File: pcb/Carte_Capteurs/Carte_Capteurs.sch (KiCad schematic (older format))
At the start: 17 parts, among them J10 Conn_01x05, J11 Conn_01x04, J12 Conn_01x04, J5 Conn_02x07_Odd_Even, J6 Molex KK 254, J7 Samtec FTS-105-01-L-DV, J8 Samtec FTS-105-01-L-DV, J9 Conn_01x05, U1 FRDM-KL25Z, U2 XBee

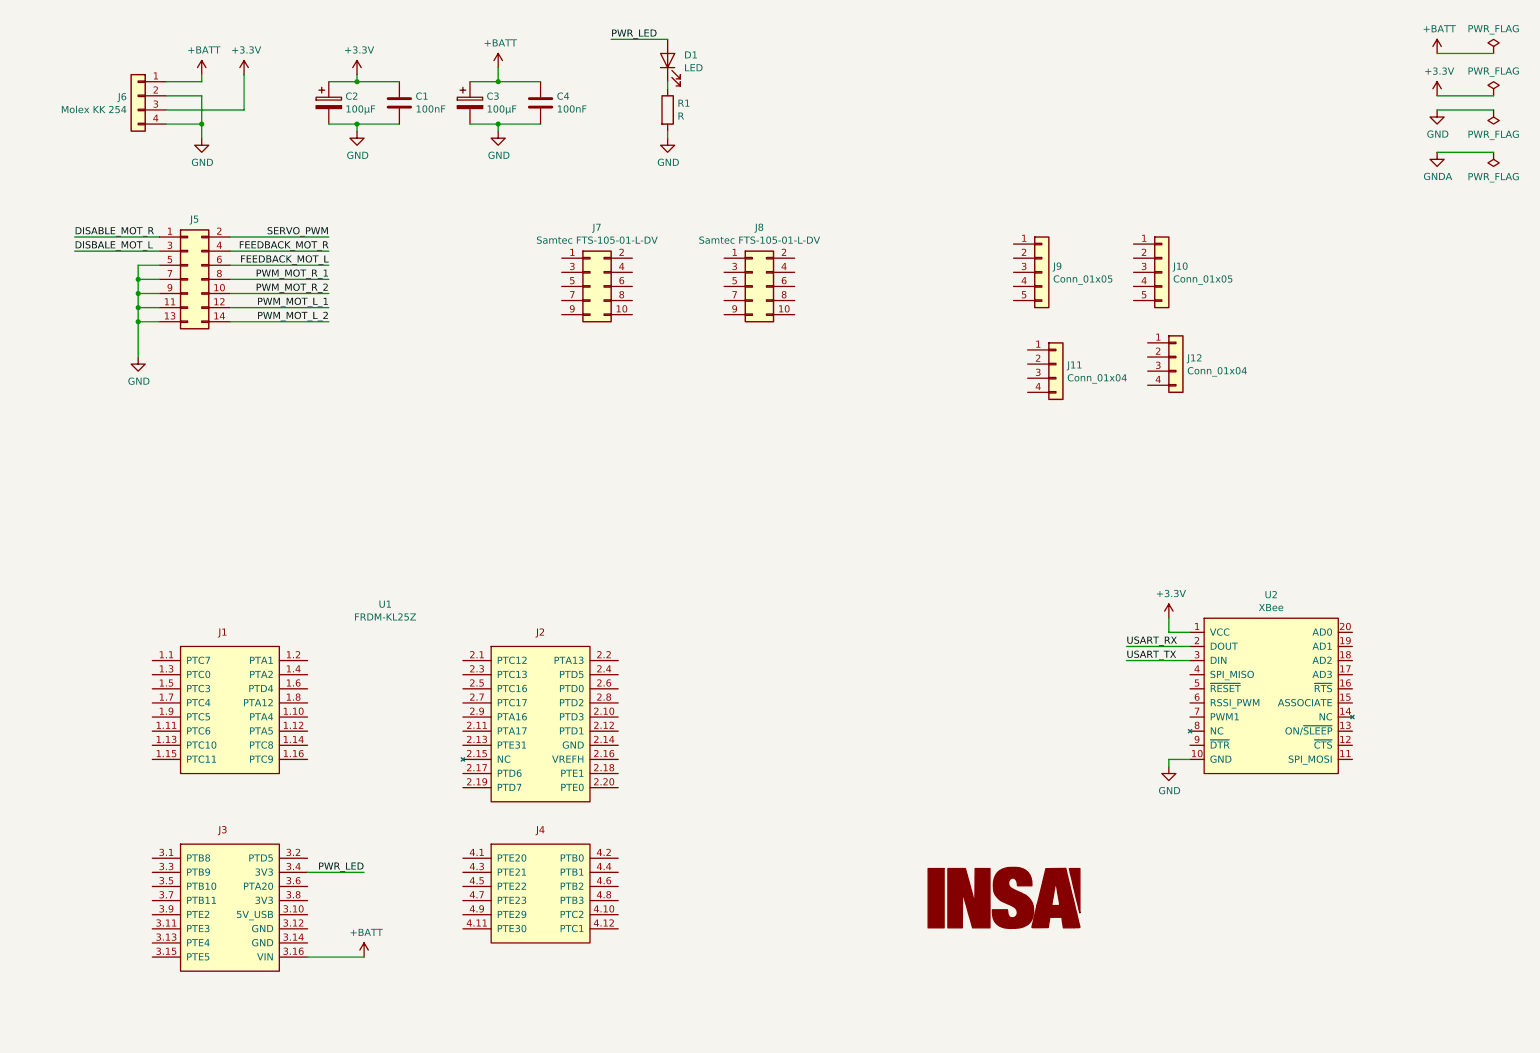
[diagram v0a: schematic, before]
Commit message: sauvegarde intermediaire
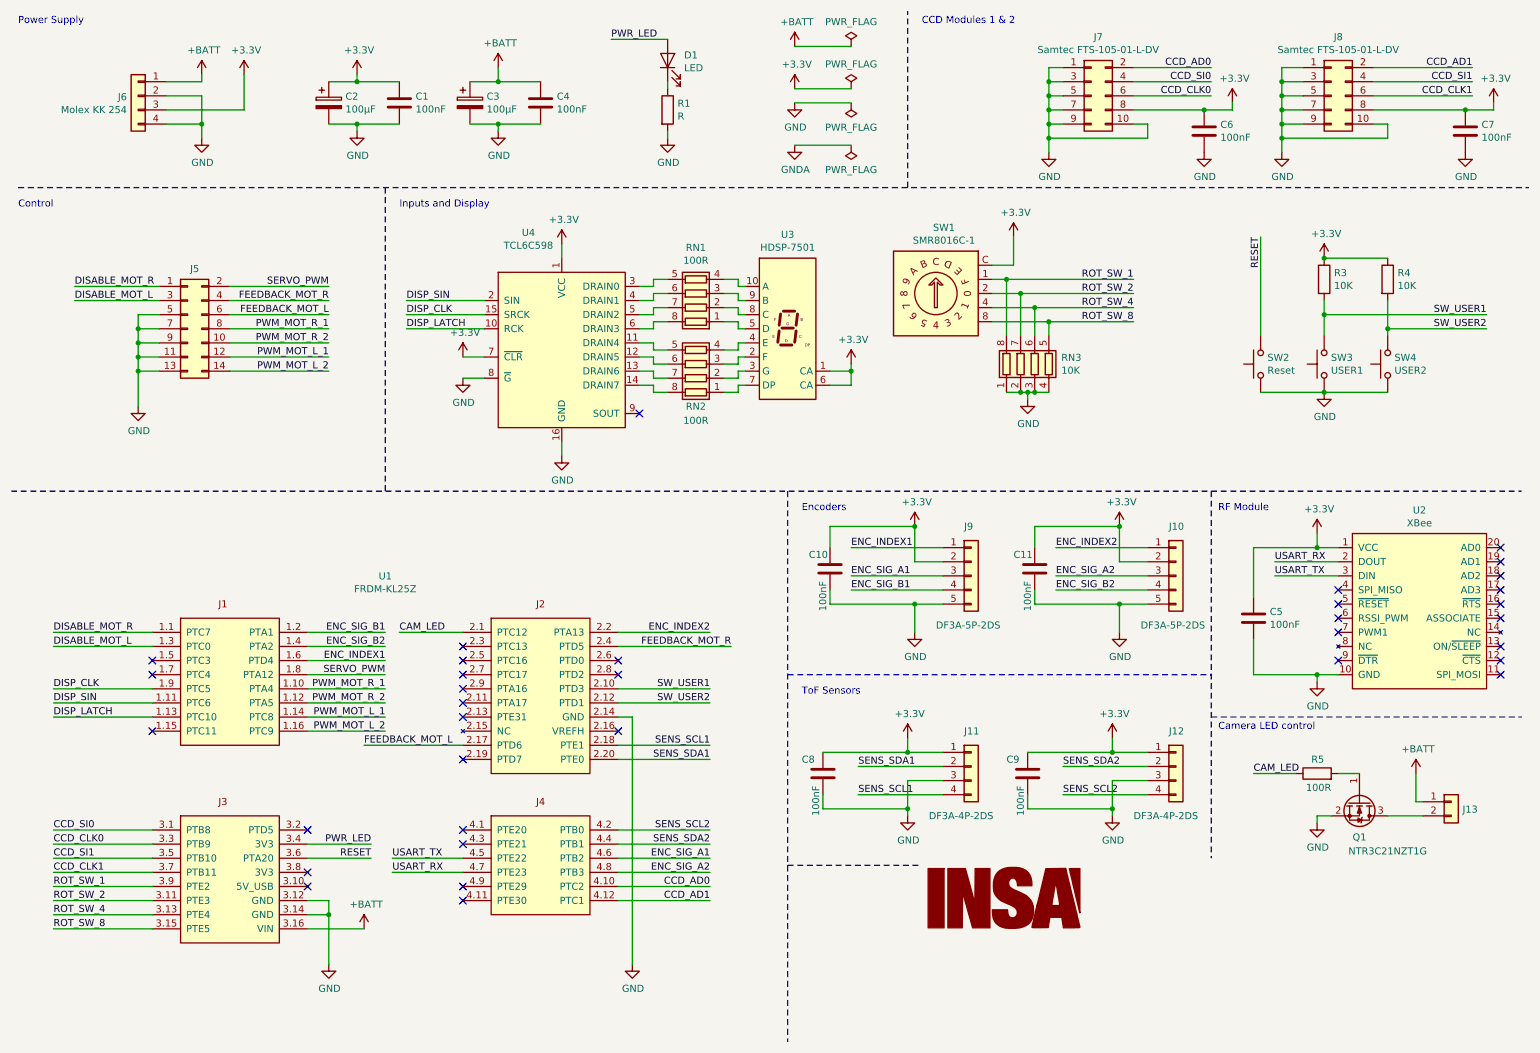
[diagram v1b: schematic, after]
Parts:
- added C10, C11, C5, C6, C7, C8, C9: 100nF, Capacitor_SMD:C_1206_3216Metric_Pad1.42x1.75mm_HandSolder, symbol Device:C
- added J13: Conn_01x02, Connector_PinHeader_2.54mm:PinHeader_1x02_P2.54mm_Vertical, symbol Connector_Generic:Conn_01x02
- added Q1: NTR3C21NZT1G, Package_TO_SOT_SMD:SOT-23, symbol Device:Q_NMOS_GSD
- added R3, R4: 10K, Resistor_SMD:R_1206_3216Metric_Pad1.42x1.75mm_HandSolder, symbol Device:R
- added R5: 100R, Resistor_SMD:R_1206_3216Metric_Pad1.42x1.75mm_HandSolder, symbol Device:R
- added RN1, RN2: 100R, Resistor_SMD:R_Array_Convex_4x1206, symbol Device:R_Pack04
- added RN3: 10K, Resistor_SMD:R_Array_Convex_4x1206, symbol Device:R_Pack04
- added SW1: SMR8016C-1, Insa:Nidec_Copal_SMR-8016C, symbol Switch:SW_Coded_SH-7050
- added SW2: Reset, Button_Switch_THT:SW_PUSH_6mm_H4.3mm, symbol Switch:SW_Push
- added SW3: USER1, Button_Switch_THT:SW_PUSH_6mm_H4.3mm, symbol Switch:SW_Push
- added SW4: USER2, Button_Switch_THT:SW_PUSH_6mm_H4.3mm, symbol Switch:SW_Push
- added U3: HDSP-7501, Display_7Segment:HDSP-A151, symbol Display_Character:HDSP-7501
- added U4: TCL6C598, Package_SO:TSSOP-16_4.4x5mm_P0.65mm, symbol Insa:TCL6C598
- J10, J9: value Conn_01x05 -> DF3A-5P-2DS; footprint Connector_PinHeader_2.54mm:PinHeader_1x05_P2.54mm_Horizontal -> Insa:DF3A-5P-2DS
- J11, J12: value Conn_01x04 -> DF3A-4P-2DS; footprint Connector_PinHeader_2.54mm:PinHeader_1x04_P2.54mm_Horizontal -> Insa:DF3A-4P-2DS
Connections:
- net DISBALE_MOT_L is gone; now on net DISABLE_MOT_L: J5.3 (Pin_3)
- net +3V3: now also J10.2 (Pin_2), J11.1 (Pin_1), J12.1 (Pin_1), J7.8 (Pin_8), J8.8 (Pin_8), J9.2 (Pin_2), C10.1, C11.1, C5.1, C6.1, C7.1, C8.1, C9.1, R3.1, R4.1, SW1.C, U3.1 (CA), U3.6 (CA), U4.1 (VCC), U4.7 (~CLR)
- net +BATT: now also J13.1 (Pin_1)
- net DISABLE_MOT_R: now also U1.1.1 (PTC7)
- net FEEDBACK_MOT_L: now also U1.2.17 (PTD6)
- net FEEDBACK_MOT_R: now also U1.2.4 (PTD5)
- net GND: now also J10.5 (Pin_5), J11.3 (Pin_3), J12.3 (Pin_3), J7.1 (Pin_1), J7.10 (Pin_10), J7.3 (Pin_3), J7.5 (Pin_5), J7.7 (Pin_7), J7.9 (Pin_9), J8.1 (Pin_1), J8.10 (Pin_10), J8.3 (Pin_3), J8.5 (Pin_5), J8.7 (Pin_7), J8.9 (Pin_9), J9.5 (Pin_5), U1.2.14 (GND), U1.3.12 (GND), U1.3.14 (GND), C10.2, C11.2, C5.2, C6.2, C7.2, C8.2, C9.2, Q1.2 (S), RN3.1 (R1.1), RN3.2 (R2.1), RN3.3 (R3.1), RN3.4 (R4.1), SW2.1, SW3.1, SW4.1, U4.16 (GND), U4.8 (~G)
- net PWM_MOT_L_1: now also U1.1.14 (PTC8)
- net PWM_MOT_L_2: now also U1.1.16 (PTC9)
- net PWM_MOT_R_1: now also U1.1.10 (PTA4)
- net PWM_MOT_R_2: now also U1.1.12 (PTA5)
- net SERVO_PWM: now also U1.1.8 (PTA12)
- net USART_RX: now also U1.4.7 (PTE23)
- net USART_TX: now also U1.4.5 (PTE22)
- net DISP_SIN: now reaches U1.1.11 (PTC6)
- net DISP_SIN: now also U4.2 (SIN)
- net DISP_LATCH: now reaches U1.1.13 (PTC10)
- net DISP_LATCH: now also U4.10 (RCK)
- net ENC_SIG_B1: now reaches U1.1.2 (PTA1)
- net ENC_SIG_B1: now also J9.4 (Pin_4)
- net DISABLE_MOT_L: now reaches U1.1.3 (PTC0)
- net ENC_SIG_B2: now reaches U1.1.4 (PTA2)
- net ENC_SIG_B2: now also J10.4 (Pin_4)
- net ENC_INDEX1: now reaches U1.1.6 (PTD4)
- net ENC_INDEX1: now also J9.1 (Pin_1)
- net DISP_CLK: now reaches U1.1.9 (PTC5)
- net DISP_CLK: now also U4.15 (SRCK)
- net CAM_LED: now reaches U1.2.1 (PTC12)
- net CAM_LED: now also R5.1
- net SW_USER1: now reaches U1.2.10 (PTD3)
- net SW_USER1: now also R3.2, SW3.2
- net SW_USER2: now reaches U1.2.12 (PTD1)
- net SW_USER2: now also R4.2, SW4.2
- net SENS_SCL1: now reaches U1.2.18 (PTE1)
- net SENS_SCL1: now also J11.4 (Pin_4)
- net ENC_INDEX2: now reaches U1.2.2 (PTA13)
- net ENC_INDEX2: now also J10.1 (Pin_1)
- net SENS_SDA1: now reaches U1.2.20 (PTE0)
- net SENS_SDA1: now also J11.2 (Pin_2)
- net CCD_SI0: now reaches U1.3.1 (PTB8)
- net CCD_SI0: now also J7.4 (Pin_4)
- net ROT_SW_2: now reaches U1.3.11 (PTE3)
- net ROT_SW_2: now also RN3.7 (R2.2), SW1.2
- net ROT_SW_4: now reaches U1.3.13 (PTE4)
- net ROT_SW_4: now also RN3.6 (R3.2), SW1.4
- net ROT_SW_8: now reaches U1.3.15 (PTE5)
- net ROT_SW_8: now also RN3.5 (R4.2), SW1.8
- net CCD_CLK0: now reaches U1.3.3 (PTB9)
- net CCD_CLK0: now also J7.6 (Pin_6)
- net CCD_SI1: now reaches U1.3.5 (PTB10)
- net CCD_SI1: now also J8.4 (Pin_4)
- net RESET: now reaches U1.3.6 (PTA20)
- net RESET: now also SW2.2
- net CCD_CLK1: now reaches U1.3.7 (PTB11)
- net CCD_CLK1: now also J8.6 (Pin_6)
- net ROT_SW_1: now reaches U1.3.9 (PTE2)
- net ROT_SW_1: now also RN3.8 (R1.2), SW1.1
- net CCD_AD0: now reaches U1.4.10 (PTC2)
- net CCD_AD0: now also J7.2 (Pin_2)
- net CCD_AD1: now reaches U1.4.12 (PTC1)
- net CCD_AD1: now also J8.2 (Pin_2)
- net SENS_SCL2: now reaches U1.4.2 (PTB0)
- net SENS_SCL2: now also J12.4 (Pin_4)
- net SENS_SDA2: now reaches U1.4.4 (PTB1)
- net SENS_SDA2: now also J12.2 (Pin_2)
- net ENC_SIG_A1: now reaches U1.4.6 (PTB2)
- net ENC_SIG_A1: now also J9.3 (Pin_3)
- net ENC_SIG_A2: now reaches U1.4.8 (PTB3)
- net ENC_SIG_A2: now also J10.3 (Pin_3)
- new net: RN1.4 (R4.1), U3.10 (A)
- new net: RN2.3 (R3.1), U3.2 (F)
- new net: RN2.2 (R2.1), U3.3 (G)
- new net: RN2.4 (R4.1), U3.4 (E)
- new net: RN1.1 (R1.1), U3.5 (D)
- new net: RN2.1 (R1.1), U3.7 (DP)
- new net: RN1.2 (R2.1), U3.8 (C)
- new net: RN1.3 (R3.1), U3.9 (B)
- new net: RN2.5 (R4.2), U4.11 (DRAIN4)
- new net: RN2.6 (R3.2), U4.12 (DRAIN5)
- new net: RN2.7 (R2.2), U4.13 (DRAIN6)
- new net: RN2.8 (R1.2), U4.14 (DRAIN7)
- new net: RN1.5 (R4.2), U4.3 (DRAIN0)
- new net: RN1.6 (R3.2), U4.4 (DRAIN1)
- new net: RN1.7 (R2.2), U4.5 (DRAIN2)
- new net: RN1.8 (R1.2), U4.6 (DRAIN3)
- new net: J13.2 (Pin_2), Q1.3 (D)
- new net: Q1.1 (G), R5.2
- no-connect marks 0 -> 35
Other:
- note added: "CCD Modules 1 & 2"
- note added: "Camera LED control"
- note added: "Control"
- note added: "Encoders"
- note added: "Inputs and Display"
- note added: "Power Supply"
- note added: "RF Module"
- note added: "ToF Sensors"
- moved on the sheet: J10, J11, J12, J5, J7, J8, J9, U1, U2
